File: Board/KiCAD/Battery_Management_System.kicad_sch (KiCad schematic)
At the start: 19 parts, among them J1 Conn_01x06_Socket, J10 Conn_01x02, J11 Conn_01x02, J12 Conn_01x02, J13 Conn_01x02, J5 Conn_01x03, J7 Conn_01x05, J8 Conn_01x02, J9 Conn_01x02

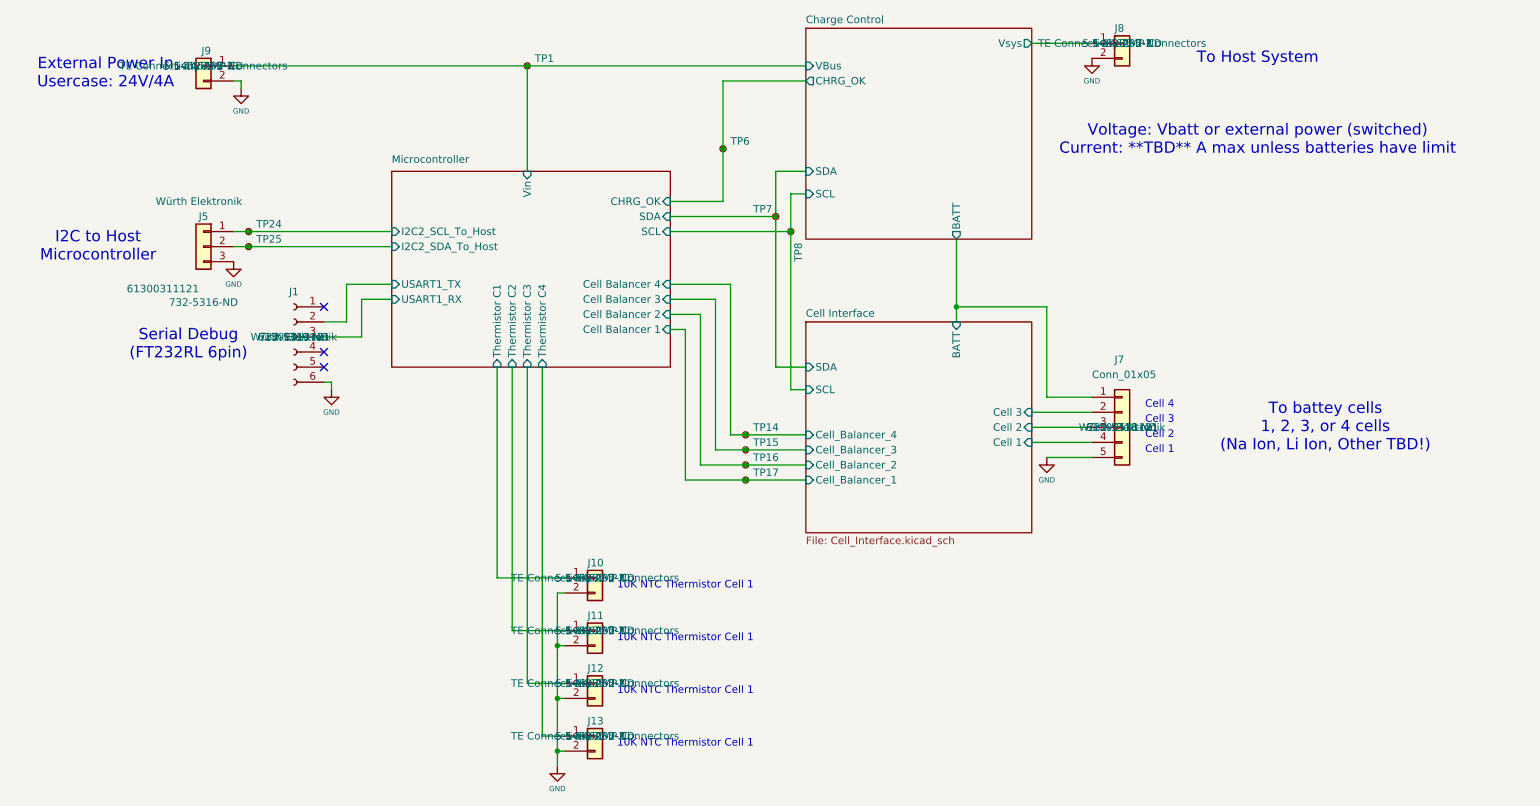
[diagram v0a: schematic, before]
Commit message: Updated schematic
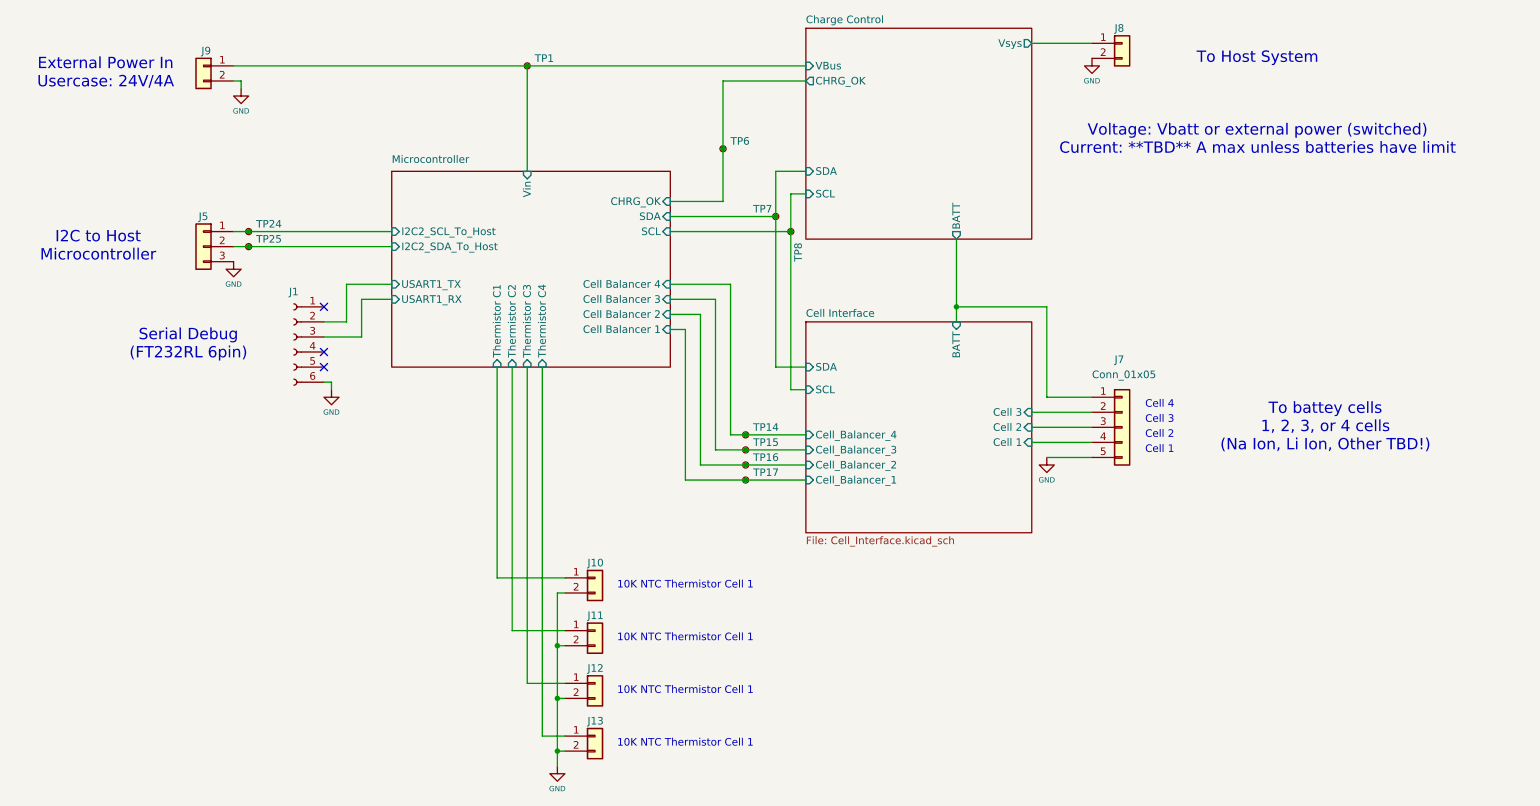
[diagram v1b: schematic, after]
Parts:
- J1: MFR Würth Elektronik -> ürth Elektronik
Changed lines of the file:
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@@
 					(size 1.27 1.27)
 				)
+				(hide yes)
 			)
 		)
@@
 					(size 1.27 1.27)
 				)
+				(hide yes)
 			)
 		)
@@
 					(size 1.27 1.27)
 				)
+				(hide yes)
 			)
 		)
@@
 					(size 1.27 1.27)
 				)
+				(hide yes)
 			)
 		)
@@
 			)
 		)
-		(property "MFR" "Würth Elektronik"
+		(property "MFR" "ürth Elektronik"
 			(at 62.23 105.41 0)
 			(effects
@@
 					(size 1.27 1.27)
 				)
+				(hide yes)
 			)
 		)
@@
 					(size 1.27 1.27)
 				)
+				(hide yes)
 			)
 		)
@@
 					(size 1.27 1.27)
 				)
+				(hide yes)
 			)
 		)
@@
 					(size 1.27 1.27)
 				)
+				(hide yes)
 			)
 		)
@@
 					(size 1.27 1.27)
 				)
+				(hide yes)
 			)
 		)
@@
 					(size 1.27 1.27)
 				)
+				(hide yes)
 			)
 		)
@@
 					(size 1.27 1.27)
 				)
+				(hide yes)
 			)
 		)
@@
 					(size 1.27 1.27)
 				)
+				(hide yes)
 			)
 		)
@@
 					(size 1.27 1.27)
 				)
+				(hide yes)
 			)
 		)
@@
 					(size 1.27 1.27)
 				)
+				(hide yes)
 			)
 		)
@@
 					(size 1.27 1.27)
 				)
+				(hide yes)
 			)
 		)
@@
 					(size 1.27 1.27)
 				)
+				(hide yes)
 			)
 		)
@@
 					(size 1.27 1.27)
 				)
+				(hide yes)
 			)
 		)
@@
 					(size 1.27 1.27)
 				)
+				(hide yes)
 			)
 		)
@@
 					(size 1.27 1.27)
 				)
+				(hide yes)
 			)
 		)
@@
 					(size 1.27 1.27)
 				)
+				(hide yes)
 			)
 		)
@@
 					(size 1.27 1.27)
 				)
+				(hide yes)
 			)
 		)
@@
 					(size 1.27 1.27)
 				)
+				(hide yes)
 			)
 		)
@@
 					(size 1.27 1.27)
 				)
+				(hide yes)
 			)
 		)
@@
 					(size 1.27 1.27)
 				)
+				(hide yes)
 			)
 		)
@@
 					(size 1.27 1.27)
 				)
+				(hide yes)
 			)
 		)
@@
 					(size 1.27 1.27)
 				)
+				(hide yes)
 			)
 		)
@@
 					(size 1.27 1.27)
 				)
-			)
-		)
+				(hide yes)
+			)
+		)
